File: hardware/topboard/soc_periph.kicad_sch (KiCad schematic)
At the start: 23 parts

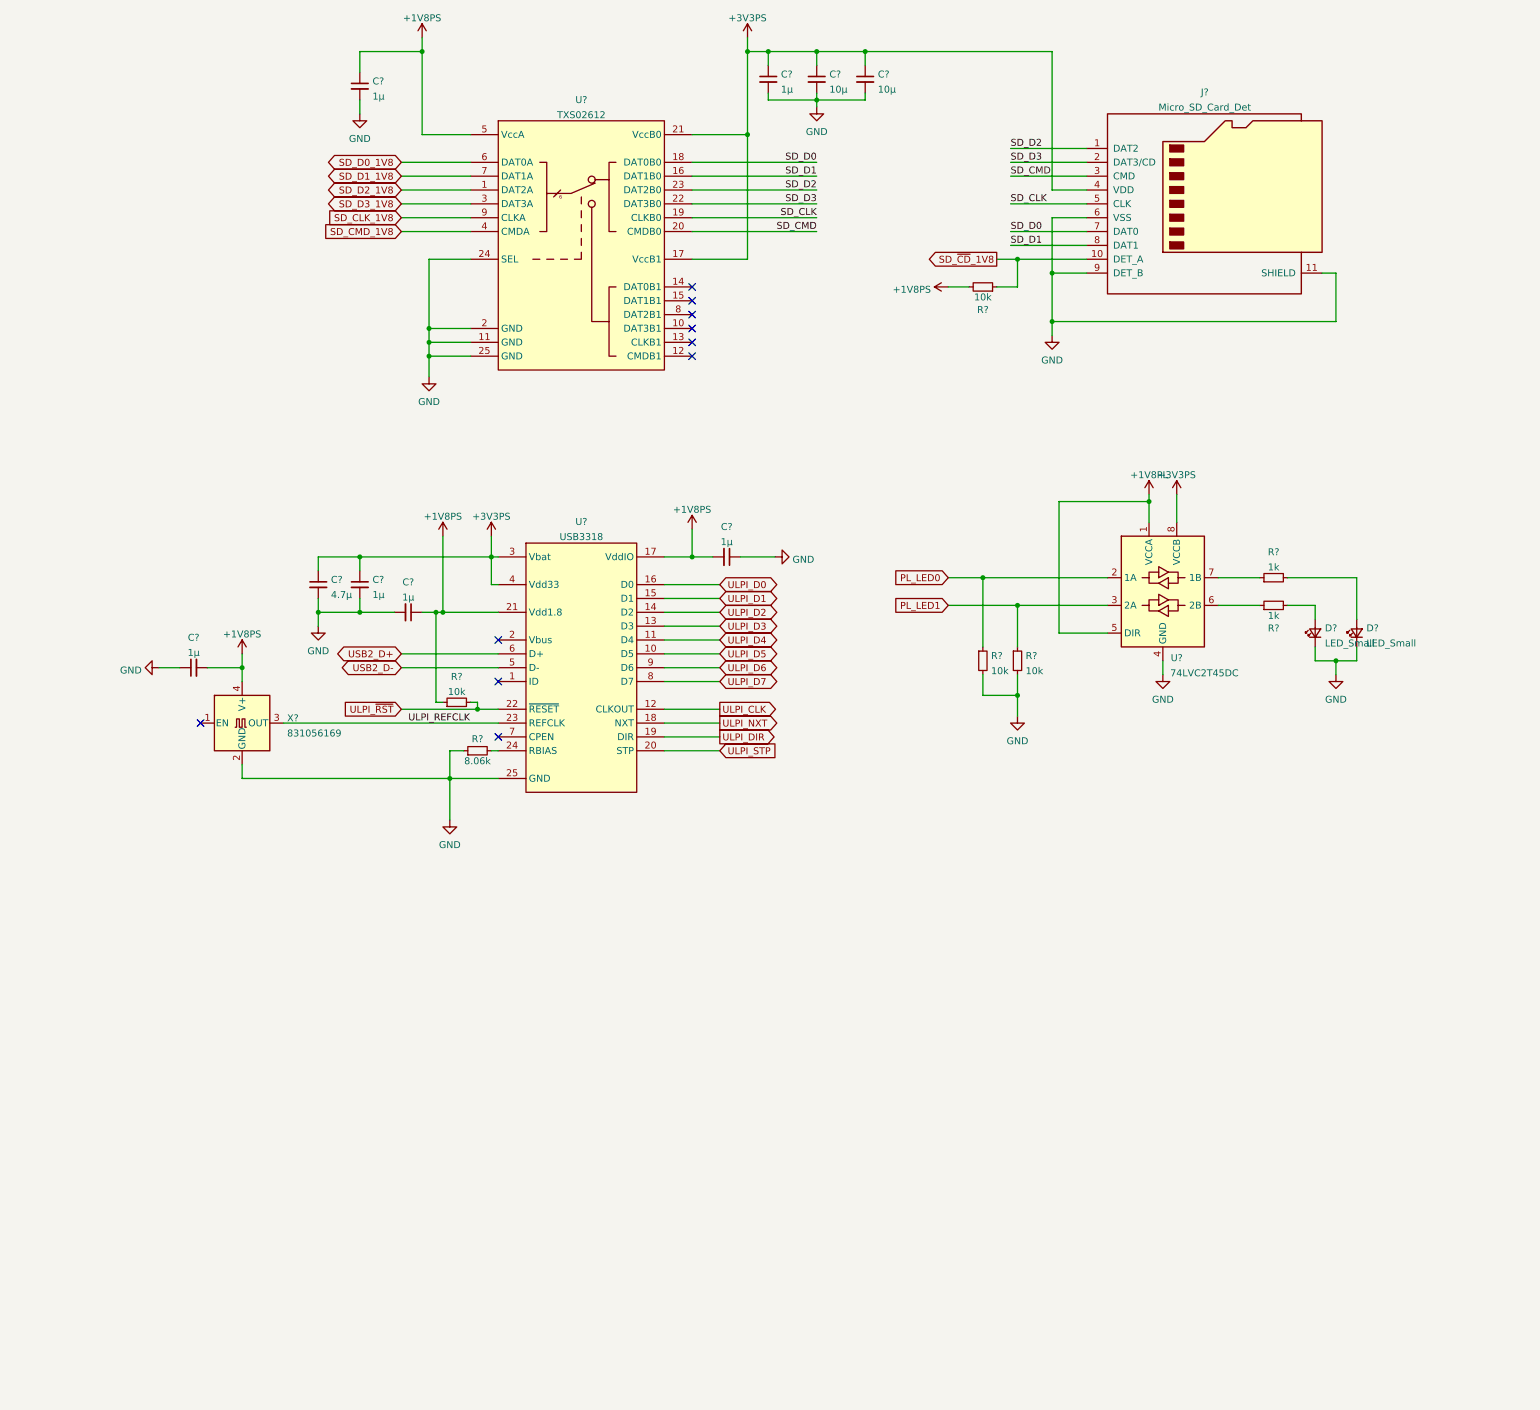
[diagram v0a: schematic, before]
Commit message: Add IMU
Signed-off-by: gatecat <gatecat@ds0.me>
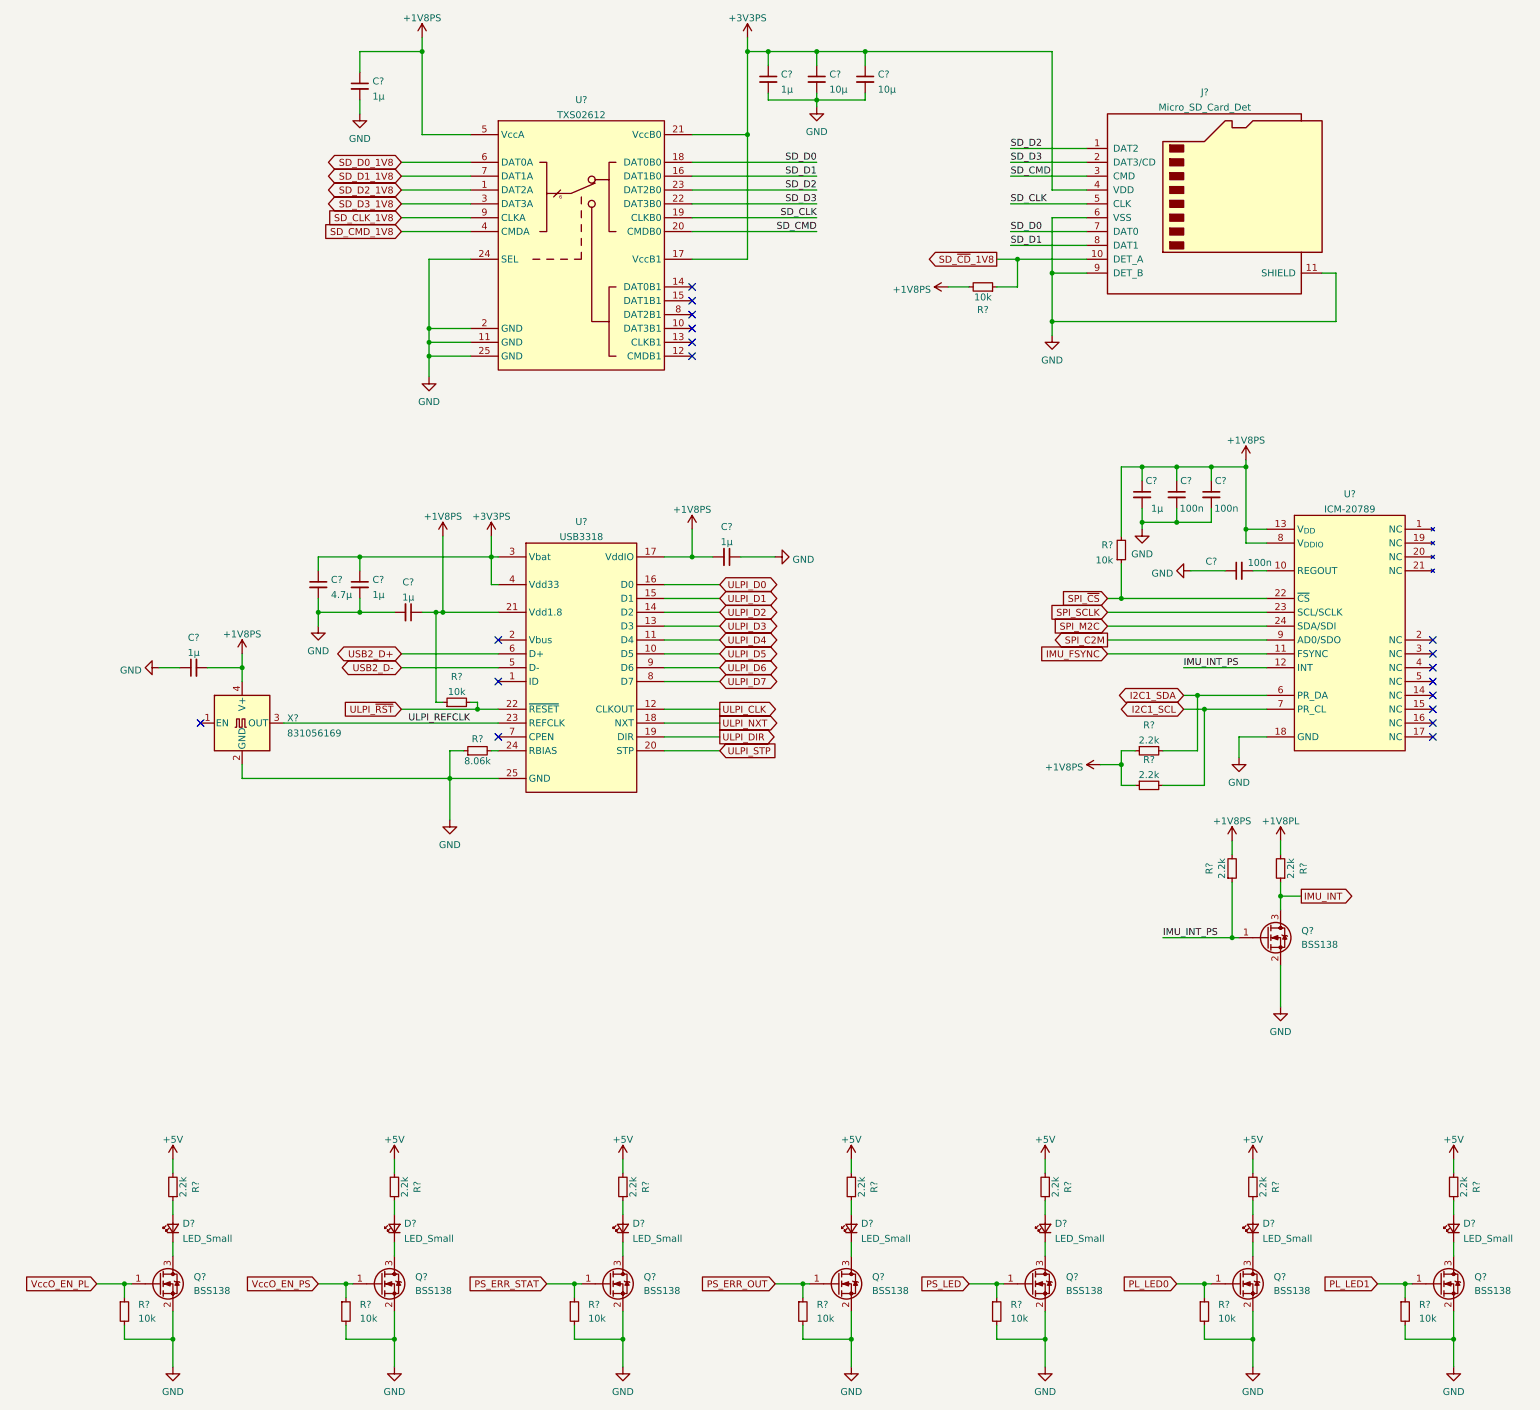
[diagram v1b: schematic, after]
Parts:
- removed D? (x2): LED_Small, symbol Device:LED_Small
- removed R? (x2): 1k, symbol Device:R_Small
- removed R? (x2): 10k, symbol Device:R_Small
- removed U?: 74LVC2T45DC, Package_SO:VSSOP-8_2.3x2mm_P0.5mm, symbol Logic_LevelTranslator:74LVC2T45DC
- added C? (x3): 100n, symbol Device:C_Small
- added C?: 1µ, symbol Device:C_Small
- added D? (x7): LED_Small, symbol Device:LED_Small
- added Q? (x8): BSS138, Package_TO_SOT_SMD:SOT-23, symbol Transistor_FET:BSS138
- added R? (x11): 2.2k, symbol Device:R_Small
- added R? (x8): 10k, symbol Device:R_Small
- added U?: ICM-20789, symbol meowality:ICM-20789
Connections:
- net +1V8PL: now also R?.2
- net +1V8PS: now also C?.1, C?.1, C?.1, R?.1, R?.1, R?.2, R?.2, U?.13 (V_{DD}), U?.8 (V_{DDIO})
- net GND: now also C?.1, C?.2, C?.2, C?.2, Q?.2 (S), Q?.2 (S), Q?.2 (S), Q?.2 (S), Q?.2 (S), Q?.2 (S), Q?.2 (S), Q?.2 (S), R?.2, R?.2, R?.2, R?.2, R?.2, R?.2, R?.2, U?.18 (GND)
- net PL_LED0: now also Q?.1 (G), R?.1
- net PL_LED1: now also Q?.1 (G), R?.1
- new net: D?.2 (A), R?.1 (x7)
- new net: C?.2, U?.10 (REGOUT)
- new net: D?.1 (K), Q?.3 (D) (x7)
- new net +5V: R?.2, R?.2, R?.2, R?.2, R?.2, R?.2, R?.2
- new net I2C1_SCL: R?.2, U?.7 (PR_CL)
- new net I2C1_SDA: R?.2, U?.6 (PR_DA)
- new net IMU_FSYNC: U?.11 (FSYNC)
- new net IMU_INT: Q?.3 (D), R?.1
- new net IMU_INT_PS: Q?.1 (G), R?.1, U?.12 (INT)
- new net PS_ERR_OUT: Q?.1 (G), R?.1
- new net PS_ERR_STAT: Q?.1 (G), R?.1
- new net PS_LED: Q?.1 (G), R?.1
- new net SPI_C2M: U?.9 (AD0/SDO)
- new net SPI_M2C: U?.24 (SDA/SDI)
- new net SPI_SCLK: U?.23 (SCL/SCLK)
- new net SPI_~{CS}: R?.1, U?.22 (~{CS})
- new net VccO_EN_PL: Q?.1 (G), R?.1
- new net VccO_EN_PS: Q?.1 (G), R?.1
- no-connect marks 10 -> 18
